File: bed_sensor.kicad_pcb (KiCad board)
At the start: 2 copper layers, 66 x 37.5 mm, 13 parts, among them J1 Conn_01x02, J2 Conn_01x06, J3 Conn_01x02, J4 Conn_01x08, Q1 2N2219, SW1 SW_SPST

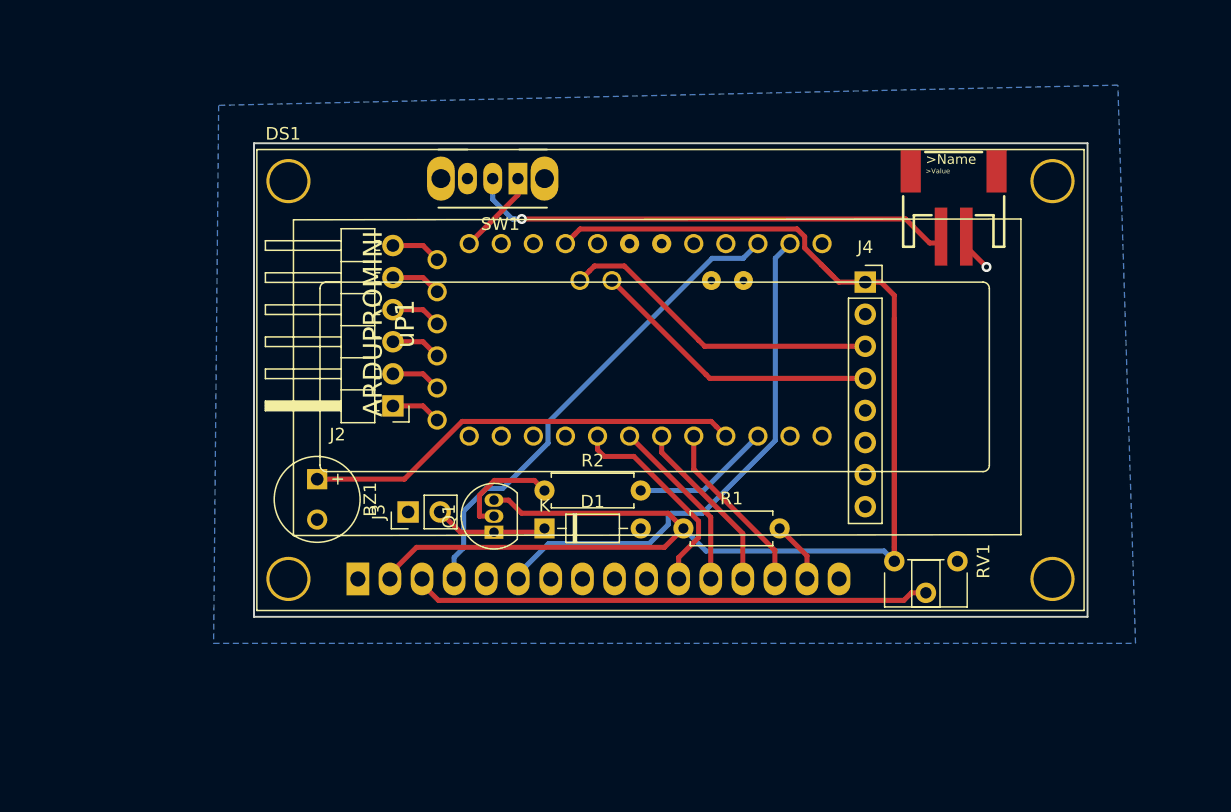
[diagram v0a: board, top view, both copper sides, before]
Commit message: fixed layout
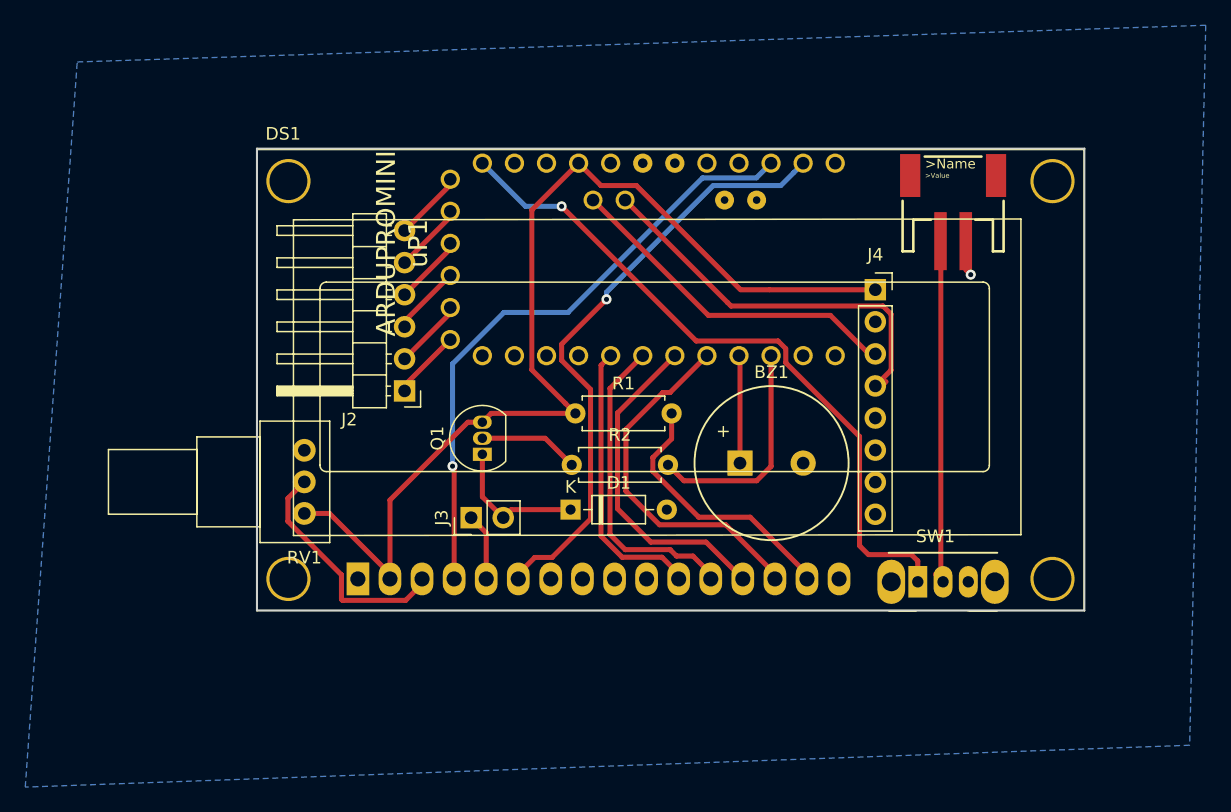
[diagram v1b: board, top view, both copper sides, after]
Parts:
- BZ1: footprint Buzzer_Beeper:MagneticBuzzer_Kingstate_KCG0601 -> components:PS1240P02BT
- RV1: footprint Potentiometer_THT:Potentiometer_ACP_CA6-H2,5_Horizontal -> Potentiometers:Potentiometer_Alps_RK09Y_Vertical
- moved RV1 52.5 mm to (163.0, 83.8), turned to 180 degrees
- moved SW1 45.0 mm to (211.6, 94.2), turned to 0 degrees
- moved BZ1 36.0 mm to (200.0, 84.8), turned to 0 degrees
- moved R1 12.5 mm to (184.4, 80.9)
- moved uP1 6.45 mm to (170.7, 78.9)
- moved Q1 6.24 mm to (177.1, 84.1)
- moved J3 5.01 mm to (176.2, 89.1)
- moved R2 2.96 mm to (184.2, 85.0)
- moved D1 2.55 mm to (184.1, 88.5)
- moved J2 1.50 mm to (170.9, 79.1)
- moved J4 1.00 mm to (208.2, 71.1)
- moved J1 0.36 mm to (214.4, 63.6)
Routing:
- net VCC: track 7.25 -> 54.9 mm, vias 0 -> 1
- net buzzer: track 54.9 -> 8.54 mm
- net +3V3: track 129.6 -> 83.3 mm
- net Net-(DS1-Pad3): track 41.1 -> 19.0 mm
- net Net-(DS1-Pad15): track 4.90 -> 21.2 mm
- net DB7: track 14.0 -> 28.6 mm
- net DB6: track 14.0 -> 26.2 mm
- net DB5: track 14.0 -> 24.9 mm
- net RS: track 38.7 -> 49.3 mm, vias 0 -> 1
- net Net-(J1-Pad1): track 39.1 -> 28.7 mm, vias 1 -> 0
- net SDA: track 23.3 -> 32.2 mm
- net E: track 41.6 -> 48.5 mm, vias 0 -> 1
- net vib: track 11.1 -> 17.9 mm
- net GND: track 2.56 -> 8.93 mm
- net DB4: track 16.6 -> 22.4 mm
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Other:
- board size 66 x 37.5 mm -> 65.5 x 36.6 mm

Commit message: updated csv
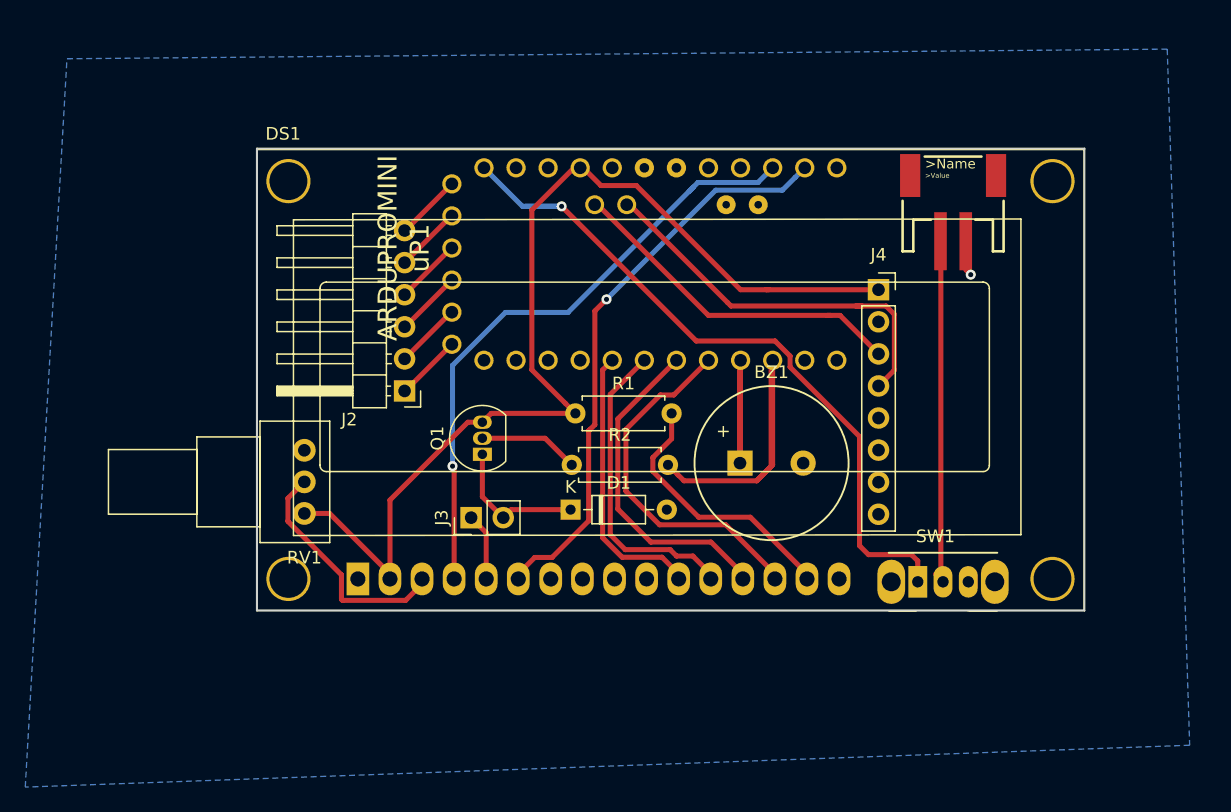
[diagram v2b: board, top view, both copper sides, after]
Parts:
- moved uP1 0.39 mm to (170.9, 79.2)
- moved J4 0.25 mm to (208.4, 71.1)
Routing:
- net vib: track 17.9 -> 28.0 mm
- net buzzer: track 8.54 -> 16.7 mm
- net VCC: track 54.9 -> 57.3 mm
- net E: track 48.5 -> 46.5 mm
- net SDA: track 32.2 -> 33.0 mm
- net +3V3: track 83.3 -> 83.9 mm
